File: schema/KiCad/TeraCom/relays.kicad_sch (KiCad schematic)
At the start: 29 parts, among them J1 Conn_01x06_Pin, J2 Screw_Terminal_01x03, J3 Screw_Terminal_01x03, J4 Screw_Terminal_01x03, J5 Screw_Terminal_01x03, K1 G5LE-1, K2 G5LE-1, K3 G5LE-1, K5 G5LE-1, U2 PC817, U3 PC817, U4 PC817, U5 PC817

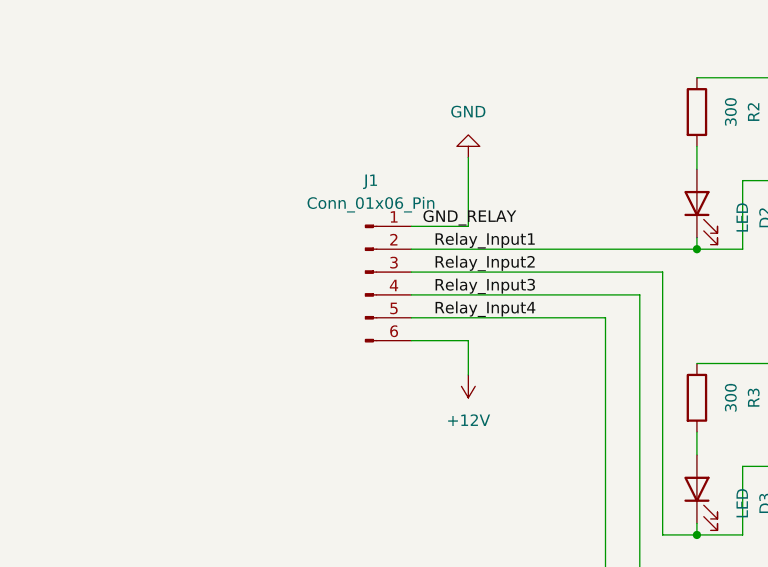
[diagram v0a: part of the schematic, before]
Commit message: v0.3
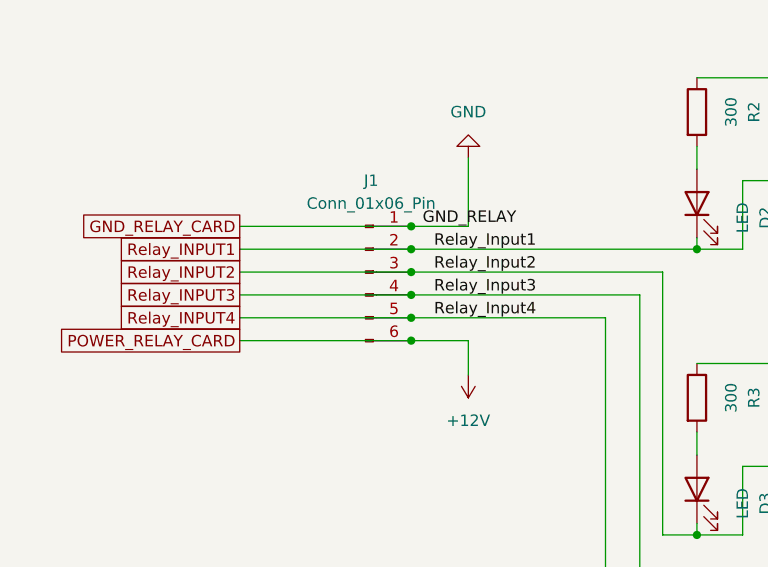
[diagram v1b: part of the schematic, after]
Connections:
- net Relay_Input1 renamed Relay_INPUT1
- net Relay_Input2 renamed Relay_INPUT2
- net Relay_Input3 renamed Relay_INPUT3
- net Relay_Input4 renamed Relay_INPUT4
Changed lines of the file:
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@@
 (kicad_sch (version 20230121) (generator eeschema)
   (paper "A4")
+  (junction (at 68.58 44.45) (diameter 0) (color 0 0 0 0)
+  )
   (junction (at 157.48 54.61) (diameter 0) (color 0 0 0 0)
   )
@@
   (junction (at 157.48 73.66) (diameter 0) (color 0 0 0 0)
   )
+  (junction (at 68.58 39.37) (diameter 0) (color 0 0 0 0)
+  )
+  (junction (at 68.58 52.07) (diameter 0) (color 0 0 0 0)
+  )
   (junction (at 114.3 86.36) (diameter 0) (color 0 0 0 0)
   )
@@
   (junction (at 100.33 137.16) (diameter 0) (color 0 0 0 0)
   )
+  (junction (at 68.58 41.91) (diameter 0) (color 0 0 0 0)
+  )
   (junction (at 157.48 86.36) (diameter 0) (color 0 0 0 0)
   )
@@
   (junction (at 157.48 41.91) (diameter 0) (color 0 0 0 0)
   )
+  (junction (at 68.58 49.53) (diameter 0) (color 0 0 0 0)
+  )
+  (junction (at 68.58 46.99) (diameter 0) (color 0 0 0 0)
+  )
   (junction (at 100.33 105.41) (diameter 0) (color 0 0 0 0)
   )
@@
     (stroke (width 0) (type default))
   )
-  (wire (pts (xy 90.17 49.53) (xy 68.58 49.53))
+  (wire (pts (xy 49.53 49.53) (xy 68.58 49.53))
     (stroke (width 0) (type default))
   )
@@
     (stroke (width 0) (type default))
   )
+  (wire (pts (xy 49.53 52.07) (xy 68.58 52.07))
+    (stroke (width 0) (type default))
+  )
   (wire (pts (xy 194.31 50.8) (xy 173.99 50.8))
     (stroke (width 0) (type default))
@@
     (stroke (width 0) (type default))
   )
+  (wire (pts (xy 49.53 39.37) (xy 68.58 39.37))
+    (stroke (width 0) (type default))
+  )
+  (wire (pts (xy 123.19 29.21) (xy 133.35 29.21))
+    (stroke (width 0) (type default))
+  )
+  (wire (pts (xy 123.19 92.71) (xy 133.35 92.71))
+    (stroke (width 0) (type default))
+  )
+  (wire (pts (xy 148.59 129.54) (xy 148.59 138.43))
+    (stroke (width 0) (type default))
+  )
+  (wire (pts (xy 152.4 137.16) (xy 157.48 137.16))
+    (stroke (width 0) (type default))
+  )
+  (wire (pts (xy 157.48 41.91) (xy 166.37 41.91))
+    (stroke (width 0) (type default))
+  )
+  (wire (pts (xy 179.07 21.59) (xy 179.07 24.13))
+    (stroke (width 0) (type default))
+  )
+  (wire (pts (xy 100.33 86.36) (xy 114.3 86.36))
+    (stroke (width 0) (type default))
+  )
+  (wire (pts (xy 49.53 44.45) (xy 68.58 44.45))
+    (stroke (width 0) (type default))
+  )
+  (wire (pts (xy 176.53 73.66) (xy 176.53 71.12))
+    (stroke (width 0) (type default))
+  )
+  (wire (pts (xy 100.33 137.16) (xy 105.41 137.16))
+    (stroke (width 0) (type default))
+  )
+  (wire (pts (xy 152.4 73.66) (xy 157.48 73.66))
+    (stroke (width 0) (type default))
+  )
+  (wire (pts (xy 194.31 124.46) (xy 194.31 114.3))
+    (stroke (width 0) (type default))
+  )
+  (wire (pts (xy 114.3 118.11) (xy 157.48 118.11))
+    (stroke (width 0) (type default))
+  )
+  (wire (pts (xy 90.17 137.16) (xy 90.17 49.53))
+    (stroke (width 0) (type default))
+  )
+  (wire (pts (xy 68.58 49.53) (xy 90.17 49.53))
+    (stroke (width 0) (type default))
+  )
+  (wire (pts (xy 194.31 129.54) (xy 191.77 129.54))
+    (stroke (width 0) (type default))
+  )
+  (wire (pts (xy 74.93 39.37) (xy 74.93 31.75))
+    (stroke (width 0) (type default))
+  )
+  (wire (pts (xy 189.23 63.5) (xy 189.23 73.66))
+    (stroke (width 0) (type default))
+  )
+  (wire (pts (xy 96.52 44.45) (xy 68.58 44.45))
+    (stroke (width 0) (type default))
+  )
   (wire (pts (xy 68.58 39.37) (xy 74.93 39.37))
     (stroke (width 0) (type default))
   )
-  (wire (pts (xy 123.19 29.21) (xy 133.35 29.21))
-    (stroke (width 0) (type default))
-  )
-  (wire (pts (xy 123.19 92.71) (xy 133.35 92.71))
-    (stroke (width 0) (type default))
-  )
-  (wire (pts (xy 148.59 129.54) (xy 148.59 138.43))
-    (stroke (width 0) (type default))
-  )
-  (wire (pts (xy 152.4 137.16) (xy 157.48 137.16))
-    (stroke (width 0) (type default))
-  )
-  (wire (pts (xy 157.48 41.91) (xy 166.37 41.91))
-    (stroke (width 0) (type default))
-  )
-  (wire (pts (xy 179.07 21.59) (xy 179.07 24.13))
-    (stroke (width 0) (type default))
-  )
-  (wire (pts (xy 100.33 86.36) (xy 114.3 86.36))
-    (stroke (width 0) (type default))
-  )
-  (wire (pts (xy 176.53 73.66) (xy 176.53 71.12))
-    (stroke (width 0) (type default))
-  )
-  (wire (pts (xy 100.33 137.16) (xy 105.41 137.16))
-    (stroke (width 0) (type default))
-  )
-  (wire (pts (xy 152.4 73.66) (xy 157.48 73.66))
-    (stroke (width 0) (type default))
-  )
-  (wire (pts (xy 194.31 124.46) (xy 194.31 114.3))
-    (stroke (width 0) (type default))
-  )
-  (wire (pts (xy 114.3 118.11) (xy 157.48 118.11))
-    (stroke (width 0) (type default))
-  )
-  (wire (pts (xy 90.17 137.16) (xy 90.17 49.53))
-    (stroke (width 0) (type default))
-  )
-  (wire (pts (xy 194.31 129.54) (xy 191.77 129.54))
-    (stroke (width 0) (type default))
-  )
-  (wire (pts (xy 74.93 39.37) (xy 74.93 31.75))
-    (stroke (width 0) (type default))
-  )
-  (wire (pts (xy 189.23 63.5) (xy 189.23 73.66))
-    (stroke (width 0) (type default))
-  )
-  (wire (pts (xy 96.52 44.45) (xy 68.58 44.45))
-    (stroke (width 0) (type default))
-  )
   (wire (pts (xy 93.98 46.99) (xy 68.58 46.99))
     (stroke (width 0) (type default))
   )
+  (wire (pts (xy 49.53 46.99) (xy 68.58 46.99))
+    (stroke (width 0) (type default))
+  )
   (wire (pts (xy 105.41 41.91) (xy 105.41 34.29))
     (stroke (width 0) (type default))
@@
   )
   (wire (pts (xy 114.3 29.21) (xy 115.57 29.21))
+    (stroke (width 0) (type default))
+  )
+  (wire (pts (xy 49.53 41.91) (xy 68.58 41.91))
     (stroke (width 0) (type default))
   )
@@
     (effects (font (size 1.27 1.27)) (justify left bottom))
   )
+  (global_label "Relay_INPUT2" (shape passive) (at 49.53 44.45 180) (fields_autoplaced)
+    (effects (font (size 1.27 1.27)) (justify right))
+    (property "Intersheetrefs" "${INTERSHEET_REFS}" (at 34.8352 44.45 0)
+      (effects (font (size 1.27 1.27)) (justify right) hide)
+    )
+  )
+  (global_label "Relay_INPUT1" (shape passive) (at 49.53 41.91 180) (fields_autoplaced)
+    (effects (font (size 1.27 1.27)) (justify right))
+    (property "Intersheetrefs" "${INTERSHEET_REFS}" (at 34.8352 41.91 0)
+      (effects (font (size 1.27 1.27)) (justify right) hide)
+    )
+  )
+  (global_label "Relay_INPUT4" (shape passive) (at 49.53 49.53 180) (fields_autoplaced)
+    (effects (font (size 1.27 1.27)) (justify right))
+    (property "Intersheetrefs" "${INTERSHEET_REFS}" (at 34.8352 49.53 0)
+      (effects (font (size 1.27 1.27)) (justify right) hide)
+    )
+  )
+  (global_label "GND_RELAY_CARD" (shape passive) (at 49.53 39.37 180) (fields_autoplaced)
+    (effects (font (size 1.27 1.27)) (justify right))
+    (property "Intersheetrefs" "${INTERSHEET_REFS}" (at 31.3275 39.37 0)
+      (effects (font (size 1.27 1.27)) (justify right) hide)
+    )
+  )
+  (global_label "Relay_INPUT3" (shape passive) (at 49.53 46.99 180) (fields_autoplaced)
+    (effects (font (size 1.27 1.27)) (justify right))
+    (property "Intersheetrefs" "${INTERSHEET_REFS}" (at 34.8352 46.99 0)
+      (effects (font (size 1.27 1.27)) (justify right) hide)
+    )
+  )
+  (global_label "POWER_RELAY_CARD" (shape passive) (at 49.53 52.07 180) (fields_autoplaced)
+    (effects (font (size 1.27 1.27)) (justify right))
+    (property "Intersheetrefs" "${INTERSHEET_REFS}" (at 28.7271 52.07 0)
+      (effects (font (size 1.27 1.27)) (justify right) hide)
+    )
+  )
   (symbol (lib_id "Device:R") (at 100.33 90.17 0) (unit 1)
